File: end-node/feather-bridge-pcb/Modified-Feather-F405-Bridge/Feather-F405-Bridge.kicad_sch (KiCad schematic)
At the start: 15 parts, among them J1 Conn_01x06, J2 Conn_01x06, J3 Conn_02x06_Odd_Even, SW1 SW_SPST, SW2 SW_SPST, U1 LoRa Radio FeatherWing, U2 NUD3112LT1, U3 NUD3112LT1

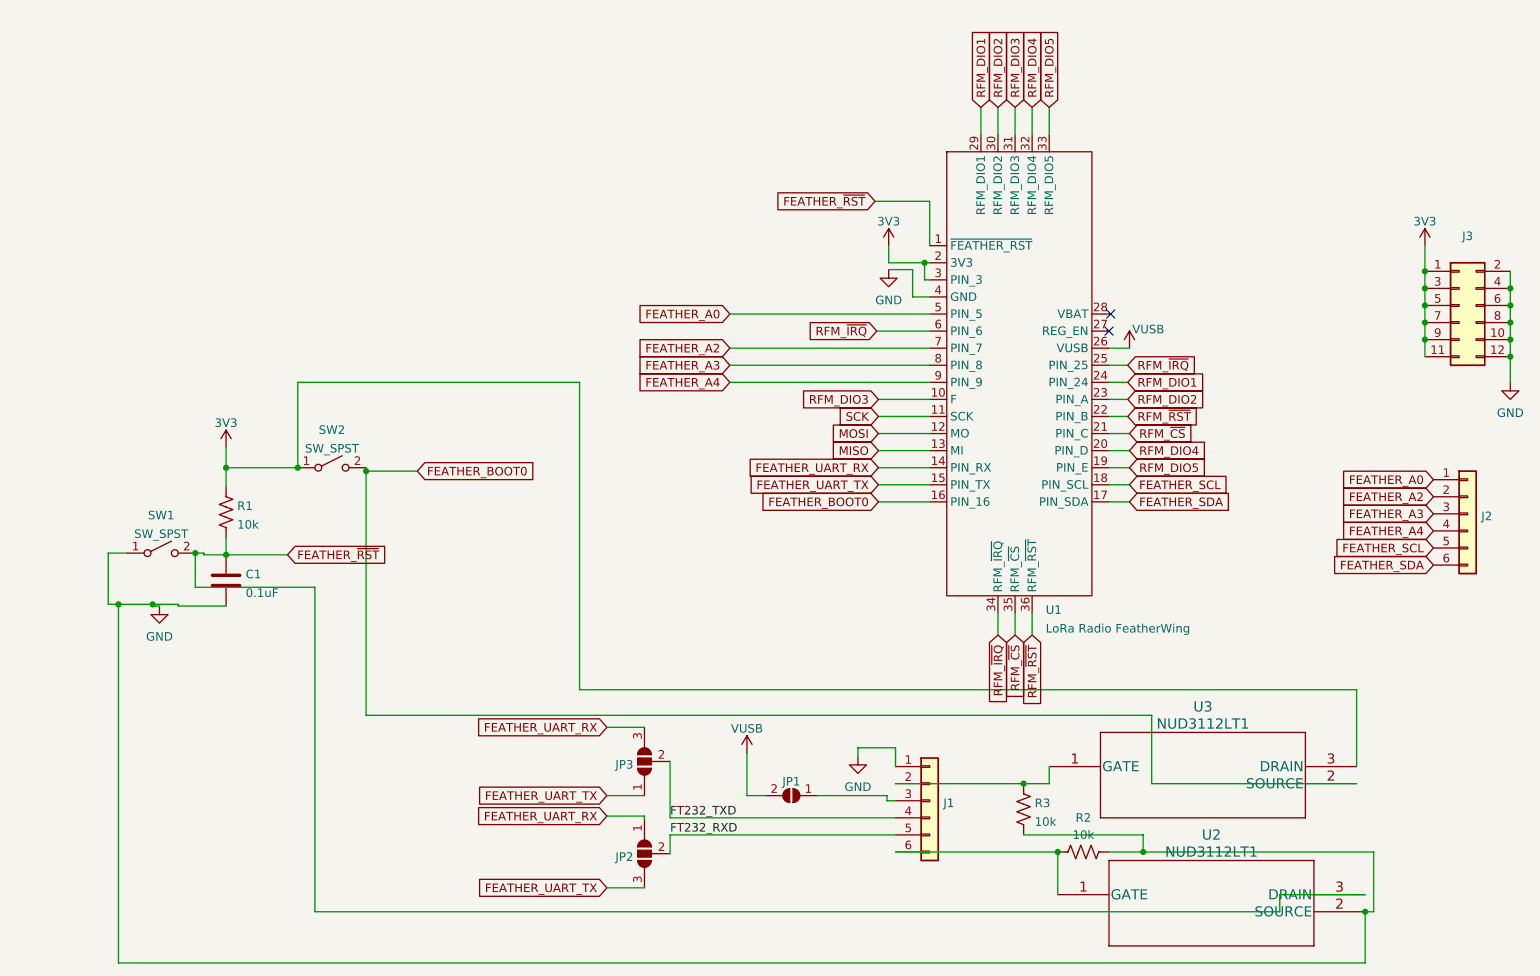
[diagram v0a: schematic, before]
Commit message: cleanup schematic
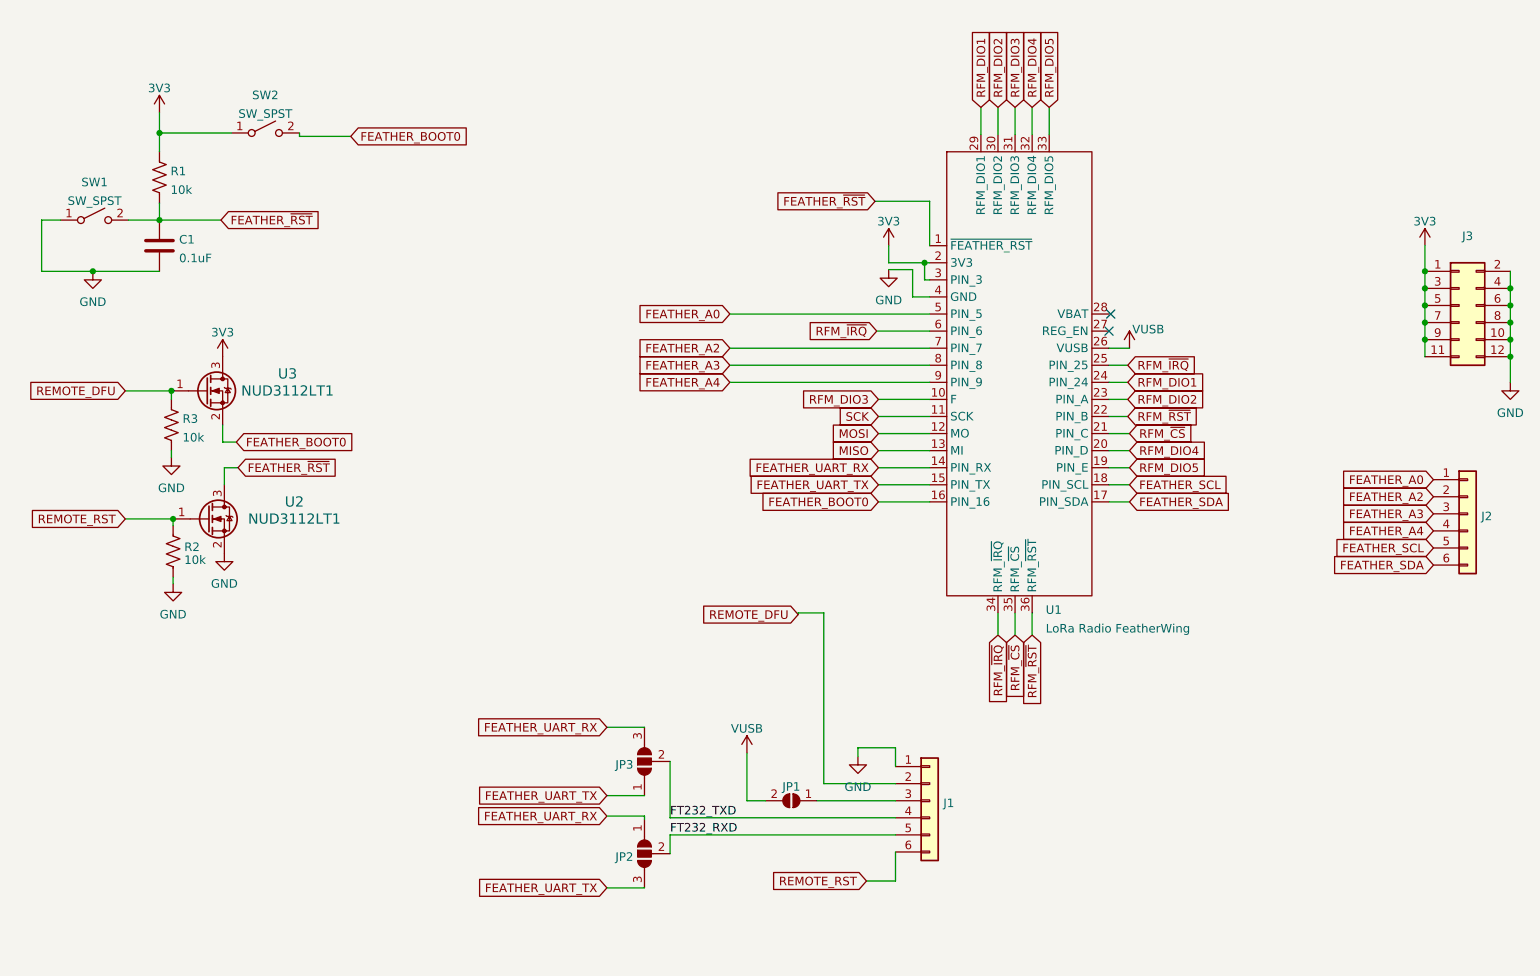
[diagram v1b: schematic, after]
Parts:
- U2, U3: footprint SOT-23_ONS -> Footprints:SOT-23; symbol 2023-04-07_15-25-17:NUD3112LT1 -> Symbols:Q_NMOS_GSD
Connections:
- net REMOTE_DFU: now reaches J1.2 (Pin_2), R3.1, U3.1 (G)
- net REMOTE_RST: now reaches J1.6 (Pin_6), R2.2, U2.1 (G)
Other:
- moved on the sheet: C1, JP1, R1, R2, R3, SW1, SW2
